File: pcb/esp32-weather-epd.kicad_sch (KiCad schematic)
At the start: 43 parts, among them J1 S2B-PH-K-S(LF)(SN), Q1 S8050, Q2 S8050, Q3 BRCS150P02ZJ, U1 CH340X, U2 TP4056X, U3 RT9080-33GJ5, U4 ESP32-WROOM-32E, U5 BME680

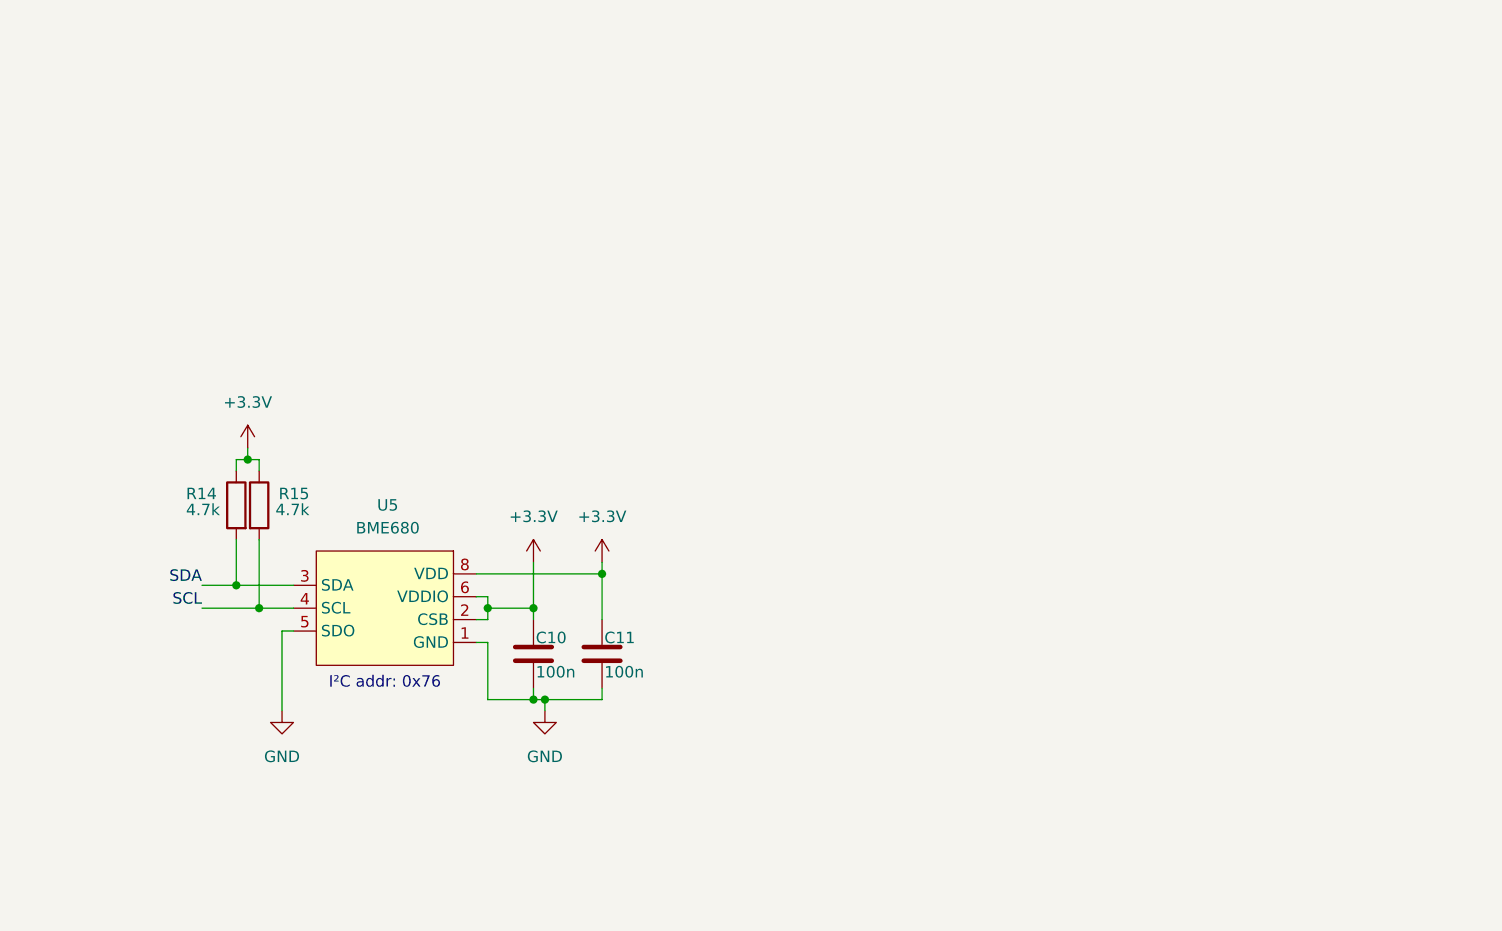
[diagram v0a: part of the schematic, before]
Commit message: fix some lib link
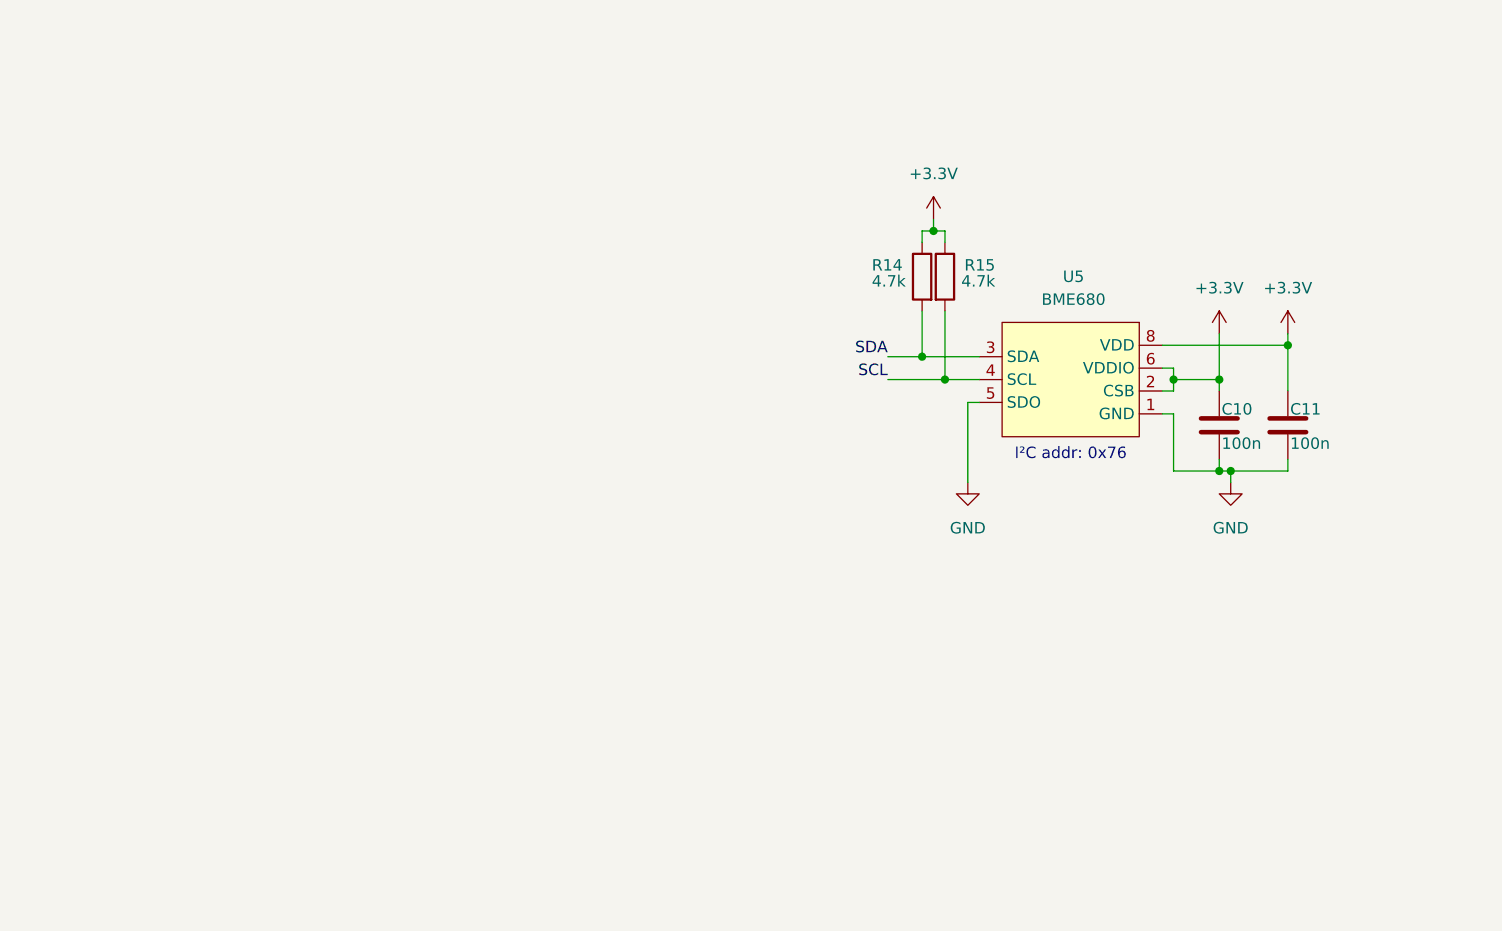
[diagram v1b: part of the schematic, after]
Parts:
- S1: footprint libs:SW-SMD_YIYUAN_YTS1C003XXX -> 0_local_lib:SW-SMD_YIYUAN_YTS1C003XXX
- U5: footprint libs:LGA-8_L3.0-W3.0-P0.80-TR -> 0_local_lib:LGA-8_L3.0-W3.0-P0.80-TR
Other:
- moved on the sheet: C10, C11, R14, R15, U5
